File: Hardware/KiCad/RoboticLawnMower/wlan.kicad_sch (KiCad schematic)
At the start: 1 part, among them U3 ESP32_NODEMCU

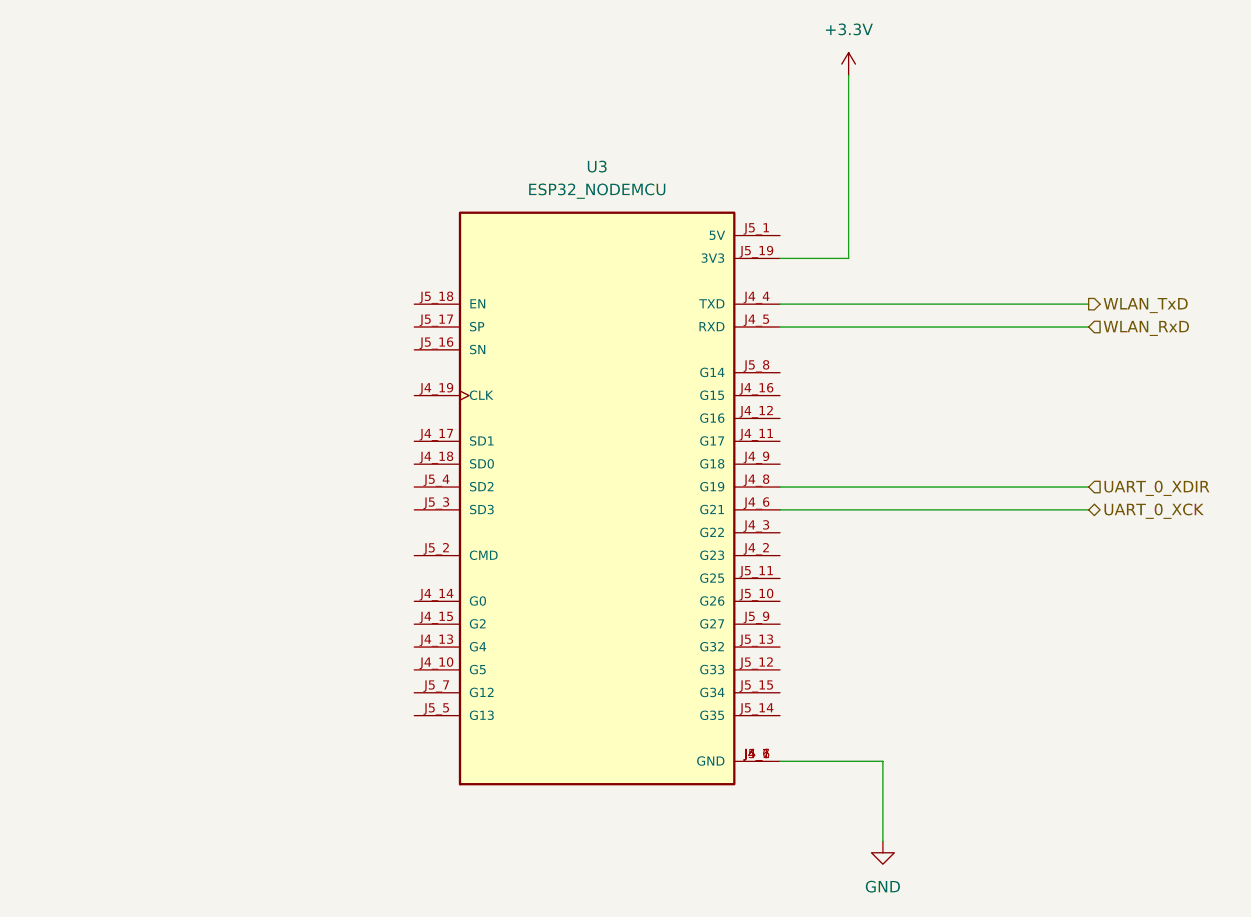
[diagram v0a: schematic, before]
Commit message: Layout
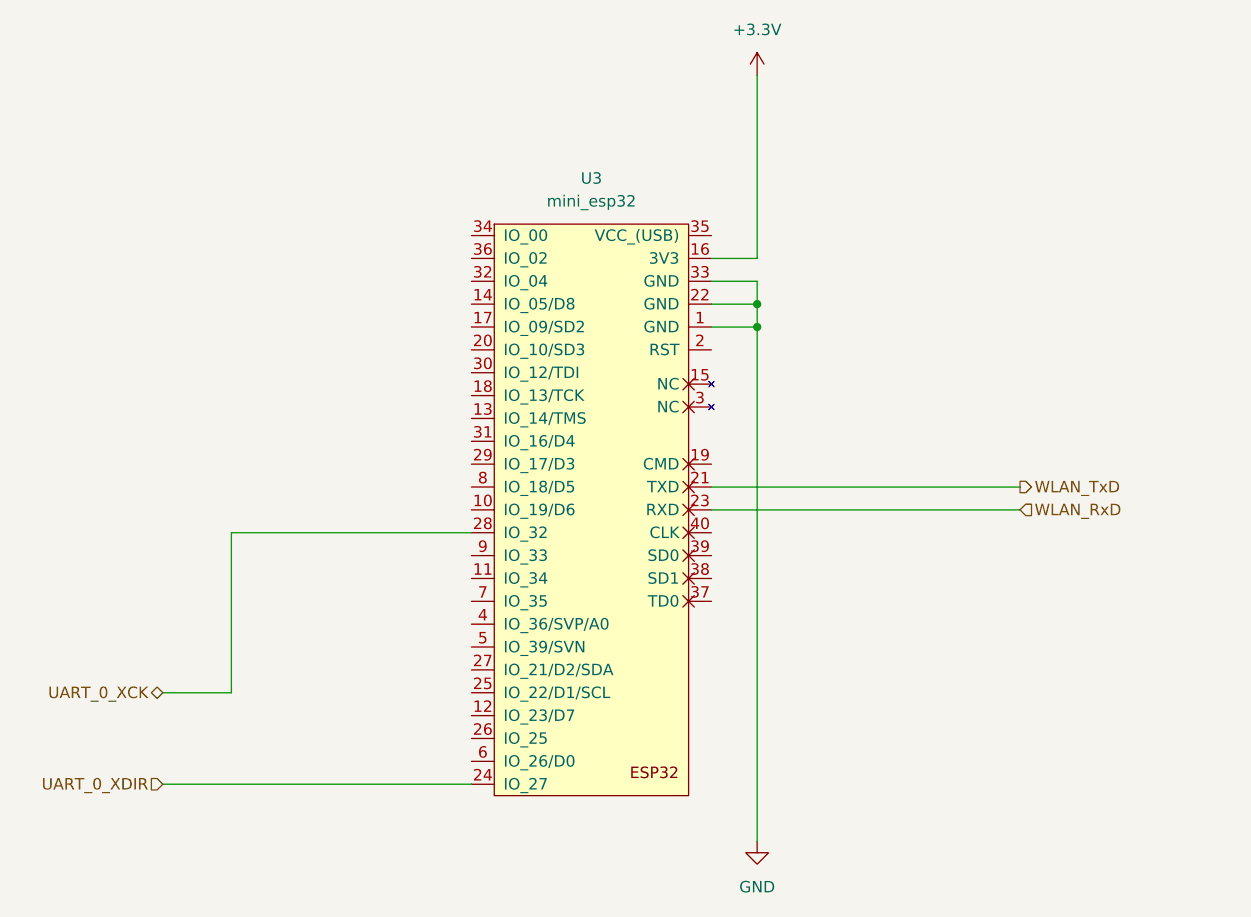
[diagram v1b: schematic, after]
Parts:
- removed U3: ESP32_NODEMCU, MODULE_ESP32_NODEMCU, symbol ESP32_NODEMCU:ESP32_NODEMCU
- added U3: mini_esp32, ESP32_mini:ESP32_mini, symbol ESP_WEMOS_D1:mini_esp32
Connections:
- net +3.3V: now also U3.16 (3V3)
- net GND: now also U3.1 (GND), U3.22 (GND), U3.33 (GND)
- net UART_0_XCK: now also U3.28 (IO_32)
- net UART_0_XDIR: now also U3.24 (IO_27)
- net WLAN_RxD: now also U3.23 (RXD)
- net WLAN_TxD: now also U3.21 (TXD)
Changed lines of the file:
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@@
 (kicad_sch (version 20211123) (generator eeschema)
   (paper "A3")
-  (wire (pts (xy 128.27 77.47) (xy 162.56 77.47))
+  (junction (at 125.73 57.15) (diameter 0) (color 0 0 0 0)
+  )
+  (junction (at 125.73 59.69) (diameter 0) (color 0 0 0 0)
+  )
+  (wire (pts (xy 93.98 110.49) (xy 59.69 110.49))
     (stroke (width 0) (type default) (color 0 0 0 0))
   )
-  (wire (pts (xy 139.7 116.84) (xy 139.7 107.95))
+  (wire (pts (xy 125.73 59.69) (xy 125.73 116.84))
     (stroke (width 0) (type default) (color 0 0 0 0))
   )
-  (wire (pts (xy 135.89 31.75) (xy 135.89 52.07))
+  (wire (pts (xy 120.65 57.15) (xy 125.73 57.15))
     (stroke (width 0) (type default) (color 0 0 0 0))
   )
-  (wire (pts (xy 128.27 80.01) (xy 162.56 80.01))
+  (wire (pts (xy 125.73 31.75) (xy 125.73 52.07))
     (stroke (width 0) (type default) (color 0 0 0 0))
   )
-  (wire (pts (xy 128.27 57.15) (xy 162.56 57.15))
+  (wire (pts (xy 67.31 82.55) (xy 93.98 82.55))
     (stroke (width 0) (type default) (color 0 0 0 0))
   )
-  (wire (pts (xy 139.7 107.95) (xy 128.27 107.95))
+  (wire (pts (xy 125.73 54.61) (xy 125.73 57.15))
     (stroke (width 0) (type default) (color 0 0 0 0))
   )
-  (wire (pts (xy 128.27 52.07) (xy 135.89 52.07))
+  (wire (pts (xy 120.65 77.47) (xy 154.94 77.47))
     (stroke (width 0) (type default) (color 0 0 0 0))
   )
-  (wire (pts (xy 128.27 59.69) (xy 162.56 59.69))
+  (wire (pts (xy 59.69 100.33) (xy 67.31 100.33))
     (stroke (width 0) (type default) (color 0 0 0 0))
   )
-  (hierarchical_label "UART_0_XDIR" (shape input) (at 162.56 77.47 0)
+  (wire (pts (xy 67.31 100.33) (xy 67.31 82.55))
+    (stroke (width 0) (type default) (color 0 0 0 0))
+  )
+  (wire (pts (xy 120.65 54.61) (xy 125.73 54.61))
+    (stroke (width 0) (type default) (color 0 0 0 0))
+  )
+  (wire (pts (xy 120.65 52.07) (xy 125.73 52.07))
+    (stroke (width 0) (type default) (color 0 0 0 0))
+  )
+  (wire (pts (xy 125.73 57.15) (xy 125.73 59.69))
+    (stroke (width 0) (type default) (color 0 0 0 0))
+  )
+  (wire (pts (xy 120.65 80.01) (xy 154.94 80.01))
+    (stroke (width 0) (type default) (color 0 0 0 0))
+  )
+  (wire (pts (xy 120.65 59.69) (xy 125.73 59.69))
+    (stroke (width 0) (type default) (color 0 0 0 0))
+  )
+  (hierarchical_label "UART_0_XDIR" (shape input) (at 59.69 110.49 180)
+    (effects (font (size 1.27 1.27)) (justify right))
+  )
+  (hierarchical_label "UART_0_XCK" (shape bidirectional) (at 59.69 100.33 180)
+    (effects (font (size 1.27 1.27)) (justify right))
+  )
+  (hierarchical_label "WLAN_RxD" (shape input) (at 154.94 80.01 0)
     (effects (font (size 1.27 1.27)) (justify left))
   )
-  (hierarchical_label "UART_0_XCK" (shape bidirectional) (at 162.56 80.01 0)
+  (hierarchical_label "WLAN_TxD" (shape output) (at 154.94 77.47 0)
     (effects (font (size 1.27 1.27)) (justify left))
   )
-  (hierarchical_label "WLAN_RxD" (shape input) (at 162.56 59.69 0)
-    (effects (font (size 1.27 1.27)) (justify left))
-  )
-  (hierarchical_label "WLAN_TxD" (shape output) (at 162.56 57.15 0)
-    (effects (font (size 1.27 1.27)) (justify left))
-  )
-  (symbol (lib_id "power:GND") (at 139.7 116.84 0) (unit 1)
+  (symbol (lib_id "ESP_WEMOS_D1:mini_esp32") (at 106.68 46.99 0) (unit 1)
     (in_bom yes) (on_board yes) (fields_autoplaced)
-    (property "Reference" "#PWR0129" (id 0) (at 139.7 123.19 0)
+    (property "Reference" "U3" (id 0) (at 107.315 43.18 0))
+    (property "Value" "mini_esp32" (id 1) (at 107.315 45.72 0))
+    (property "Footprint" "ESP32_mini:ESP32_mini" (id 2) (at 110.49 44.45 0)
       (effects (font (size 1.27 1.27)) hide)
     )
-    (property "Value" "GND" (id 1) (at 139.7 121.92 0))
-    (property "Footprint" "" (id 2) (at 139.7 116.84 0)
+    (property "Datasheet" "" (id 3) (at 110.49 44.45 0)
       (effects (font (size 1.27 1.27)) hide)
     )
-    (property "Datasheet" "" (id 3) (at 139.7 116.84 0)
+    (pin "1")
+    (pin "2")
+    (pin "3")
+    (pin "4")
+    (pin "5")
+    (pin "10")
+    (pin "11")
+    (pin "12")
+    (pin "13")
+    (pin "14")
+    (pin "15")
+    (pin "16")
+    (pin "17")
+    (pin "18")
+    (pin "19")
+    (pin "20")
+    (pin "21")
+    (pin "22")
+    (pin "23")
+    (pin "24")
+    (pin "25")
+    (pin "26")
+    (pin "27")
+    (pin "28")
+    (pin "29")
+    (pin "30")
+    (pin "31")
+    (pin "32")
+    (pin "33")
+    (pin "34")
+    (pin "35")
+    (pin "36")
+    (pin "37")
+    (pin "38")
+    (pin "39")
+    (pin "40")
+    (pin "6")
+    (pin "7")
+    (pin "8")
+    (pin "9")
+  )
+  (symbol (lib_id "power:GND") (at 125.73 116.84 0) (unit 1)
+    (in_bom yes) (on_board yes) (fields_autoplaced)
+    (property "Reference" "#PWR0129" (id 0) (at 125.73 123.19 0)
+      (effects (font (size 1.27 1.27)) hide)
+    )
+    (property "Value" "GND" (id 1) (at 125.73 121.92 0))
+    (property "Footprint" "" (id 2) (at 125.73 116.84 0)
+      (effects (font (size 1.27 1.27)) hide)
+    )
+    (property "Datasheet" "" (id 3) (at 125.73 116.84 0)
       (effects (font (size 1.27 1.27)) hide)
     )
     (pin "1")
   )
-  (symbol (lib_id "power:+3.3V") (at 135.89 31.75 0) (unit 1)
+  (symbol (lib_id "power:+3.3V") (at 125.73 31.75 0) (unit 1)
     (in_bom yes) (on_board yes) (fields_autoplaced)
-    (property "Reference" "#PWR0130" (id 0) (at 135.89 35.56 0)
+    (property "Reference" "#PWR0130" (id 0) (at 125.73 35.56 0)
       (effects (font (size 1.27 1.27)) hide)
     )
-    (property "Value" "+3.3V" (id 1) (at 135.89 26.67 0))
-    (property "Footprint" "" (id 2) (at 135.89 31.75 0)
+    (property "Value" "+3.3V" (id 1) (at 125.73 26.67 0))
+    (property "Footprint" "" (id 2) (at 125.73 31.75 0)
       (effects (font (size 1.27 1.27)) hide)
     )
-    (property "Datasheet" "" (id 3) (at 135.89 31.75 0)
+    (property "Datasheet" "" (id 3) (at 125.73 31.75 0)
       (effects (font (size 1.27 1.27)) hide)
     )
     (pin "1")
   )
-  (symbol (lib_id "ESP32_NODEMCU:ESP32_NODEMCU") (at 107.95 77.47 0) (unit 1)
-    (in_bom yes) (on_board yes) (fields_autoplaced)
-    (property "Reference" "U3" (id 0) (at 107.95 41.91 0))
-    (property "Value" "ESP32_NODEMCU" (id 1) (at 107.95 44.45 0))
-    (property "Footprint" "MODULE_ESP32_NODEMCU" (id 2) (at 107.95 77.47 0)
-      (effects (font (size 1.27 1.27)) (justify bottom) hide)
-    )
-    (property "Datasheet" "" (id 3) (at 107.95 77.47 0)
-      (effects (font (size 1.27 1.27)) hide)
-    )
-    (property "STANDARD" "Manufacturer Recommendations" (id 4) (at 107.95 77.47 0)
-      (effects (font (size 1.27 1.27)) (justify bottom) hide)
-    )
-    (property "MANUFACTURER" "Espressif" (id 5) (at 107.95 77.47 0)
-      (effects (font (size 1.27 1.27)) (justify bottom) hide)
-    )
-    (property "MAXIMUM_PACKAGE_HEIGHT" "6.6 mm" (id 6) (at 107.95 77.47 0)
-      (effects (font (size 1.27 1.27)) (justify bottom) hide)
-    )
-    (pin "J4_1")
-    (pin "J4_10")
-    (pin "J4_11")
-    (pin "J4_12")
-    (pin "J4_13")
-    (pin "J4_14")
-    (pin "J4_15")
-    (pin "J4_16")
-    (pin "J4_17")
-    (pin "J4_18")
-    (pin "J4_19")
-    (pin "J4_2")
-    (pin "J4_3")
-    (pin "J4_4")
-    (pin "J4_5")
-    (pin "J4_6")
-    (pin "J4_7")
-    (pin "J4_8")
-    (pin "J4_9")
-    (pin "J5_1")
-    (pin "J5_10")
-    (pin "J5_11")
-    (pin "J5_12")
-    (pin "J5_13")
-    (pin "J5_14")
-    (pin "J5_15")
-    (pin "J5_16")
-    (pin "J5_17")
-    (pin "J5_18")
-    (pin "J5_19")
-    (pin "J5_2")
-    (pin "J5_3")
-    (pin "J5_4")
-    (pin "J5_5")
-    (pin "J5_6")
-    (pin "J5_7")
-    (pin "J5_8")
-    (pin "J5_9")
-  )
 )
